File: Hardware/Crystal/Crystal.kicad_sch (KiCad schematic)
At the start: 48 parts, among them J1 USB_B_Micro, U1 AP63205WU, U2 NCP1117-3.3_SOT223, U3 ESP32-C3-WROOM-02, U4 TXS0102DCT, U5 TXS0108EPW

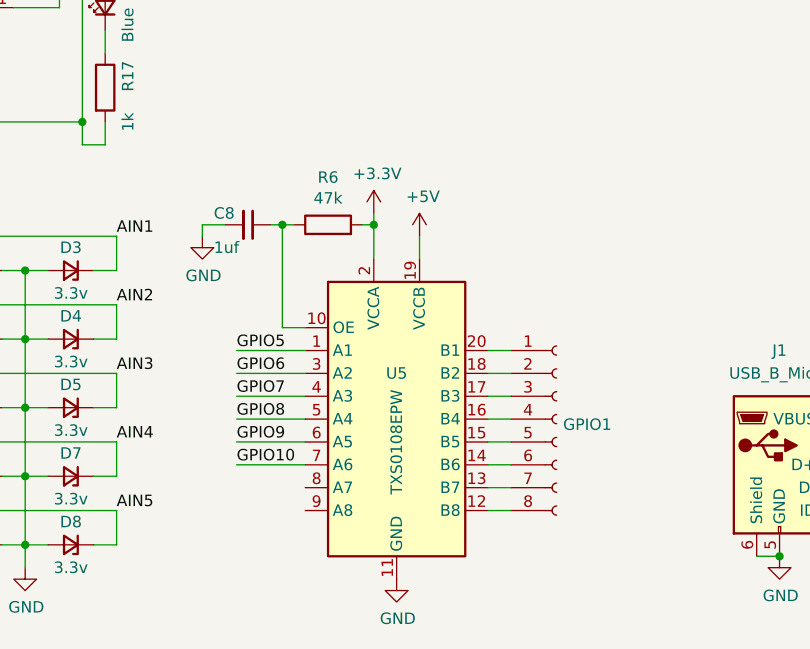
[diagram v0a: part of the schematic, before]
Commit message: Further board cleanup
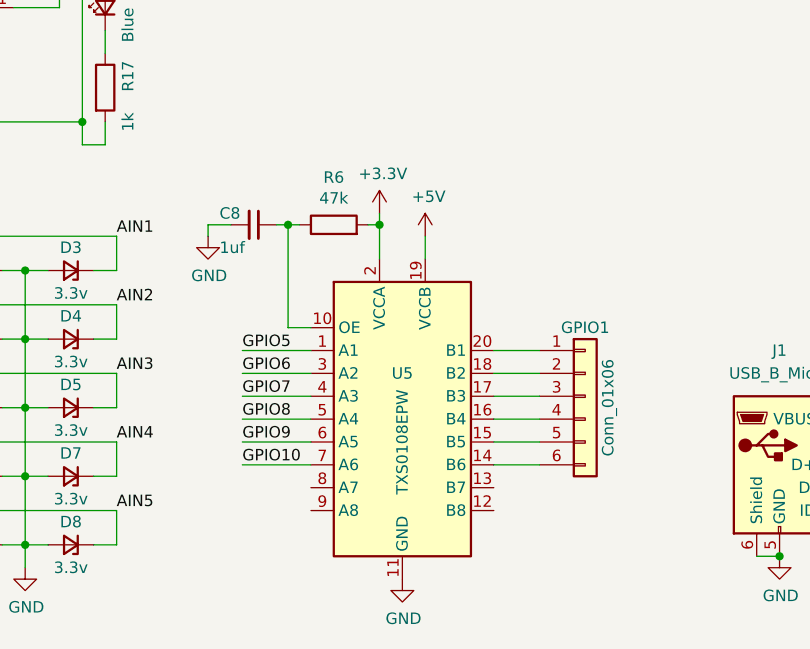
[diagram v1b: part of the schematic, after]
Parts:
- removed GPIO1: Conn_01x08_Female, Connector_PinSocket_2.54mm:PinSocket_1x08_P2.54mm_Vertical, symbol ESP32-C3 WIFI-rescue:Conn_01x08_Female-Connector
- added GPIO1: Conn_01x06, Connector_PinSocket_2.54mm:PinSocket_1x06_P2.54mm_Vertical, symbol Connector_Generic:Conn_01x06
- BOOT1, RESET1: footprint Button_Switch_SMD:SW_SPST_B3U-3000P -> Button_Switch_SMD:SW_SPST_B3U-3000P-B
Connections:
- net at U5.14 (B6): now also GPIO1.6 (Pin_6)
- net at U5.15 (B5): now also GPIO1.5 (Pin_5)
- net at U5.16 (B4): now also GPIO1.4 (Pin_4)
- net at U5.17 (B3): now also GPIO1.3 (Pin_3)
- net at U5.18 (B2): now also GPIO1.2 (Pin_2)
- net at U5.20 (B1): now also GPIO1.1 (Pin_1)
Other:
- moved on the sheet: C8, R6, U5
